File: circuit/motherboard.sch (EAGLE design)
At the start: 3 parts

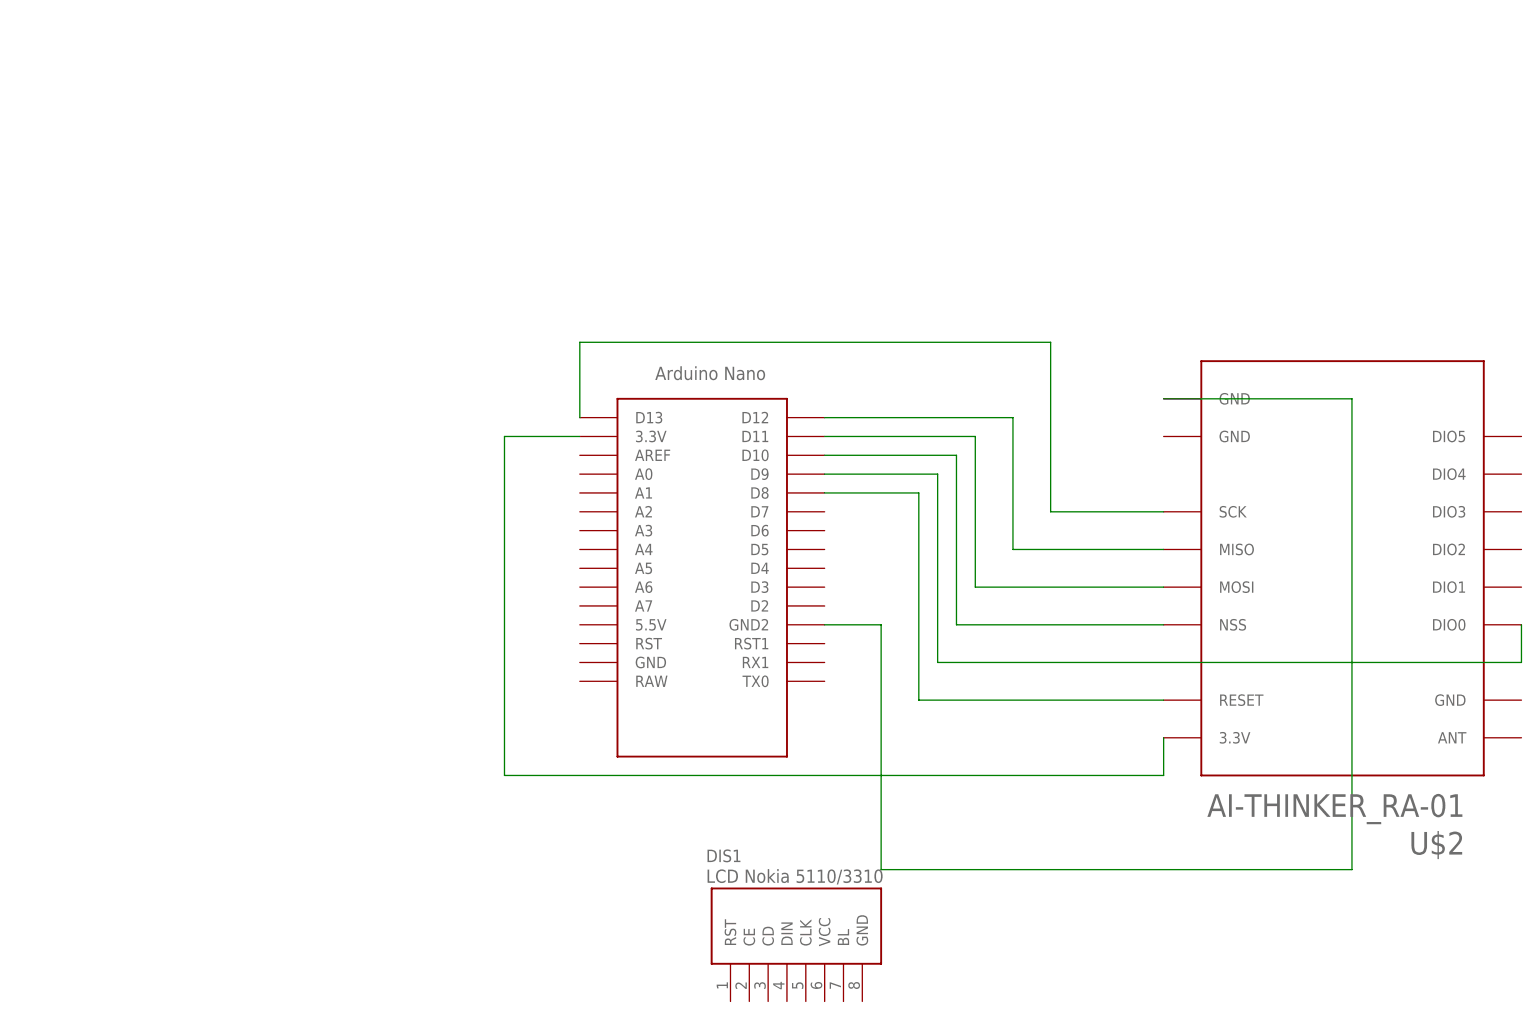
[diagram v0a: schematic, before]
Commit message: Think I've got the circuitry down, boarding next
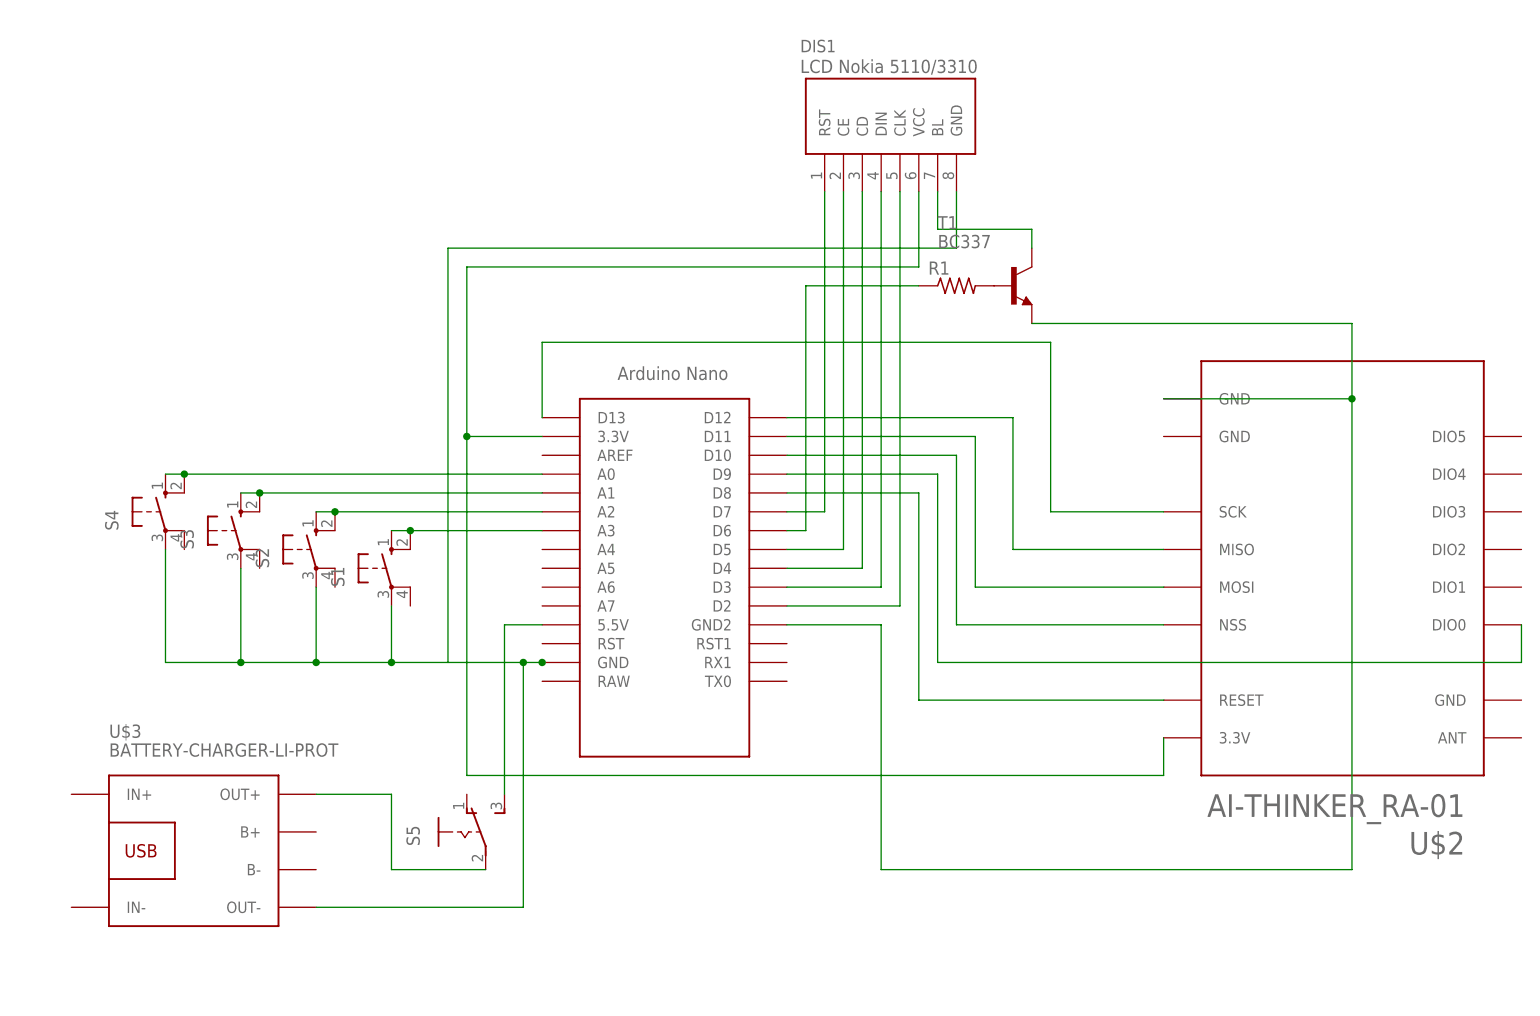
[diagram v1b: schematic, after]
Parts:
- added R1: (no value), adafruit:FLIPFLOP-RES
- added S1, S2, S3, S4: (no value), switch-omron:10-XX
- added S5: (no value), switch:255SB
- added T1: BC337, transistor:BC337
- added U$3: BATTERY-CHARGER-LI-PROT, diy-modules:BATTERY-CHARGER-LI-PROT
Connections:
- new net N$10: DIS1.DIN, U$1.D3
- new net N$11: DIS1.CD, U$1.D4
- new net N$12: DIS1.CE, U$1.D5
- new net N$13: DIS1.RST, U$1.D7
- new net N$14: R1.1, U$1.D6
- new net N$15: S5.P, U$3.OUT+
- new net N$16: R1.2, T1.B
- new net N$17: DIS1.BL, T1.C
- new net N$18: S4.S, S4.S1, U$1.A0
- new net N$19: S3.S, S3.S1, U$1.A1
- new net N$20: S2.S, S2.S1, U$1.A2
- new net N$21: S1.S, S1.S1, U$1.A3
- new net N$22: DIS1.GND, S1.P, S2.P, S3.P, S4.P, U$1.GND, U$3.OUT-
- new net N$23: S5.S, U$1.5.5V
- new net N$9: DIS1.CLK, U$1.D2
- net N$1: now also DIS1.VCC
- net N$3: now also T1.E
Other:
- moved on the sheet: DIS1

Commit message: PCB coming along nicely
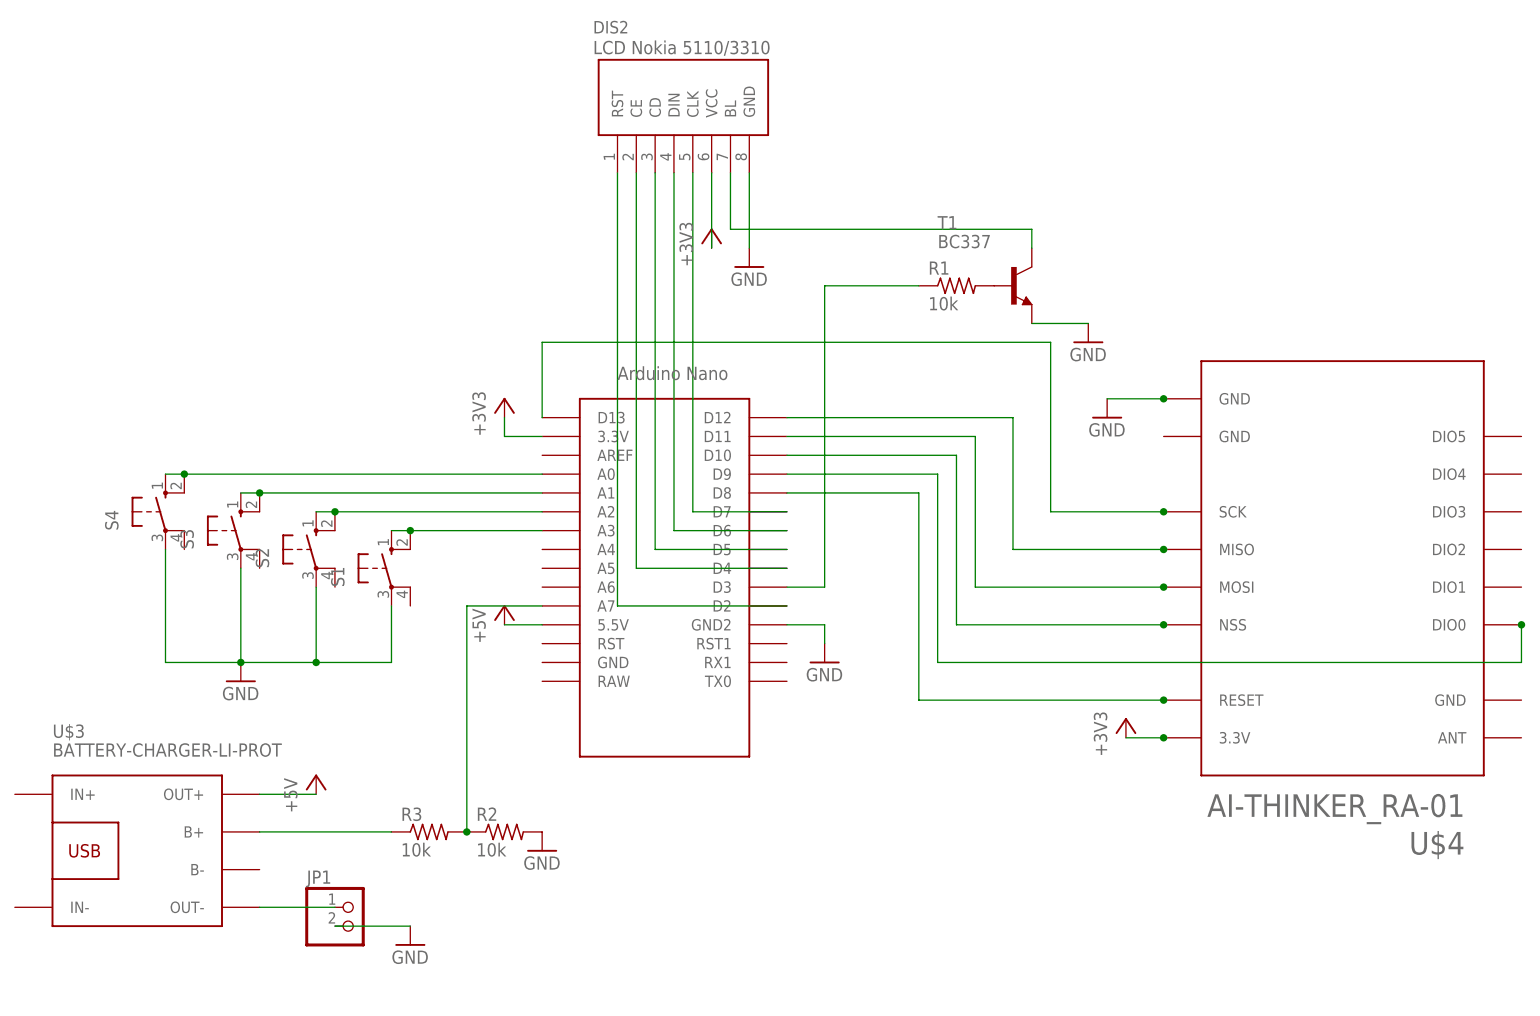
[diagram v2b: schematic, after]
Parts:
- removed DIS1: NOKIA5110, _LCD_Nokia5110:NOKIA5110
- removed S5: (no value), switch:255SB
- removed U$2: AI-THINKER_RA-01, LoRa_modules:AI-THINKER_RA-01
- added DIS2: NOKIA5110, _LCD_Nokia5110-minimal:NOKIA5110
- added JP1: (no value), pinhead:PINHD-1X2/90
- added R2, R3: 10k, adafruit:FLIPFLOP-RES
- added U$4: AI-THINKER_RA-01, lora-ra-02-minimal-because-labels-fuckup-rotating:AI-THINKER_RA-01
- R1: value (none) -> 10k
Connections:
- removed net N$14: R1.1, U$1.D6
- removed net N$15: S5.P, U$3.OUT+
- removed net N$22: DIS1.GND, S1.P, S2.P, S3.P, S4.P, U$1.GND, U$3.OUT-
- removed net N$23: S5.S, U$1.5.5V
- new net +3V3: DIS2.VCC, U$1.3.3V, U$4.3.3V
- new net +5V: U$1.5.5V, U$3.OUT+
- new net GND: DIS2.GND, JP1.2, R2.2, S1.P, S2.P, S3.P, S4.P, T1.E, U$1.GND2, U$4.GND@2
- new net N$24: R2.1, R3.2, U$1.A7
- new net N$25: R3.1, U$3.B+
- net N$1: now also JP1.1, U$3.OUT-; no longer DIS1.VCC, U$1.3.3V, U$2.3.3V
- net N$10: now also DIS2.DIN, U$1.D6; no longer DIS1.DIN, U$1.D3
- net N$11: now also DIS2.CD, U$1.D5; no longer DIS1.CD, U$1.D4
- net N$12: now also DIS2.CE, U$1.D4; no longer DIS1.CE, U$1.D5
- net N$13: now also R1.1, U$1.D3; no longer DIS1.RST, U$1.D7
- net N$17: now also DIS2.BL; no longer DIS1.BL
- net N$2: now also U$4.SCK; no longer U$2.SCK
- net N$3: now also DIS2.CLK, U$1.D7; no longer T1.E, U$1.GND2, U$2.GND@2
- net N$4: now also U$4.MISO; no longer U$2.MISO
- net N$5: now also U$4.MOSI; no longer U$2.MOSI
- net N$6: now also U$4.NSS; no longer U$2.NSS
- net N$7: now also U$4.DIO0; no longer U$2.DIO0
- net N$8: now also U$4.RESET; no longer U$2.RESET
- net N$9: now also DIS2.RST; no longer DIS1.CLK
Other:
- moved on the sheet: U$3
